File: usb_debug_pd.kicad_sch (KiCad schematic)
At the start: 85 parts, among them J4 Tag-Connect_TC2050-IDC-NL_2x5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, J7 USB-C_Kycon_KUSBX-SL2-CS1N24-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, Q12 DMG1012T-7, Q3 DMG1012T-7, U29 W25Q80DV_USON, U30 TPS65988DHRSHR, U31 NTS0102_XSON, U32 NCP730BMT330_WSON, U34 FT230X_QFN, U40 AP22615A_TSOT26, U42 TPD4E05U06QDQARQ1

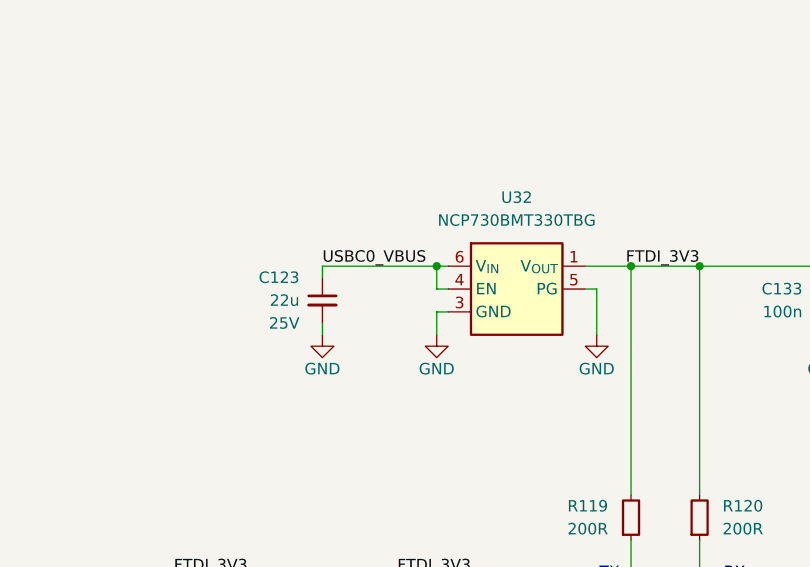
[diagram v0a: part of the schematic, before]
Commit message: [#85488] After rebase cleanup
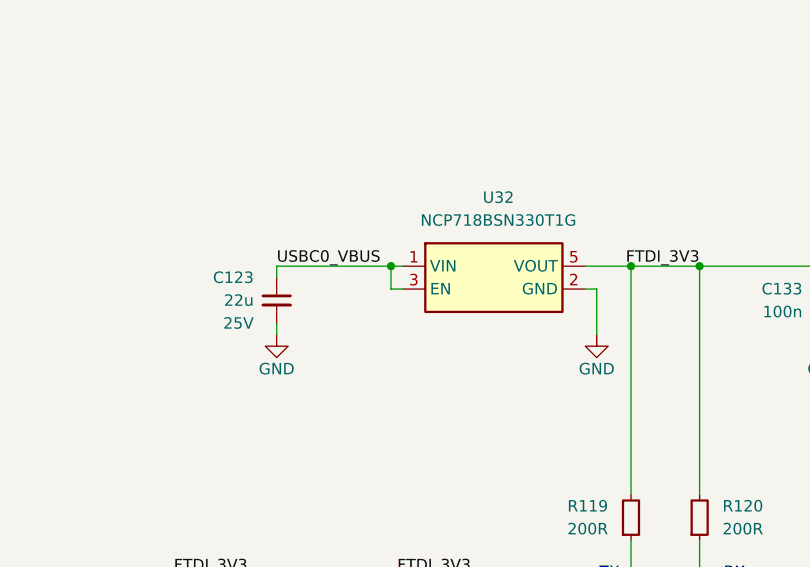
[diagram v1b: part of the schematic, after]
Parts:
- U32: value NCP730BMT330_WSON -> NCP718BSN330T1G; footprint antmicro-footprints:WSON-6-1EP_2x2mm_P0.65mm -> antmicro-footprints:SOT-23-5; symbol antmicroPMICVoltageRegulatorsLinear:NCP730BMT330_WSON -> antmicroPMICVoltageRegulatorsLinear:NCP718BSN330T1G; MPN NCP730BMT330TBG -> NCP718BSN330T1G
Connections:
- net FTDI_3V3: now also U32.5 (VOUT); no longer U32.1 (V_{OUT})
- net GND: now also U32.2 (GND); no longer U32.3 (GND), U32.5 (PG), U32.7 (GND)
- net USBC0_VBUS: now also U32.1 (VIN), U32.3 (EN); no longer U32.4 (EN), U32.6 (V_{IN})
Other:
- moved on the sheet: C123
